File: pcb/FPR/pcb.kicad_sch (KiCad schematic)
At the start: 52 parts, among them J1 Conn_01x03_Male, J12 V Solar, J13 V batt, J2 Conn_01x03_Male, J3 Conn_01x03_Male, J4 Conn_01x03_Male, J5 Conn_01x04_Female, J6 SD Card Reader, J7 cell power headers, J8 cell data headers, U1 ATmega328-P, U2 LM2574HVM-12, U3 LT3650EMSE-8.4-PBF, U4 LM311, Y1 16MHz

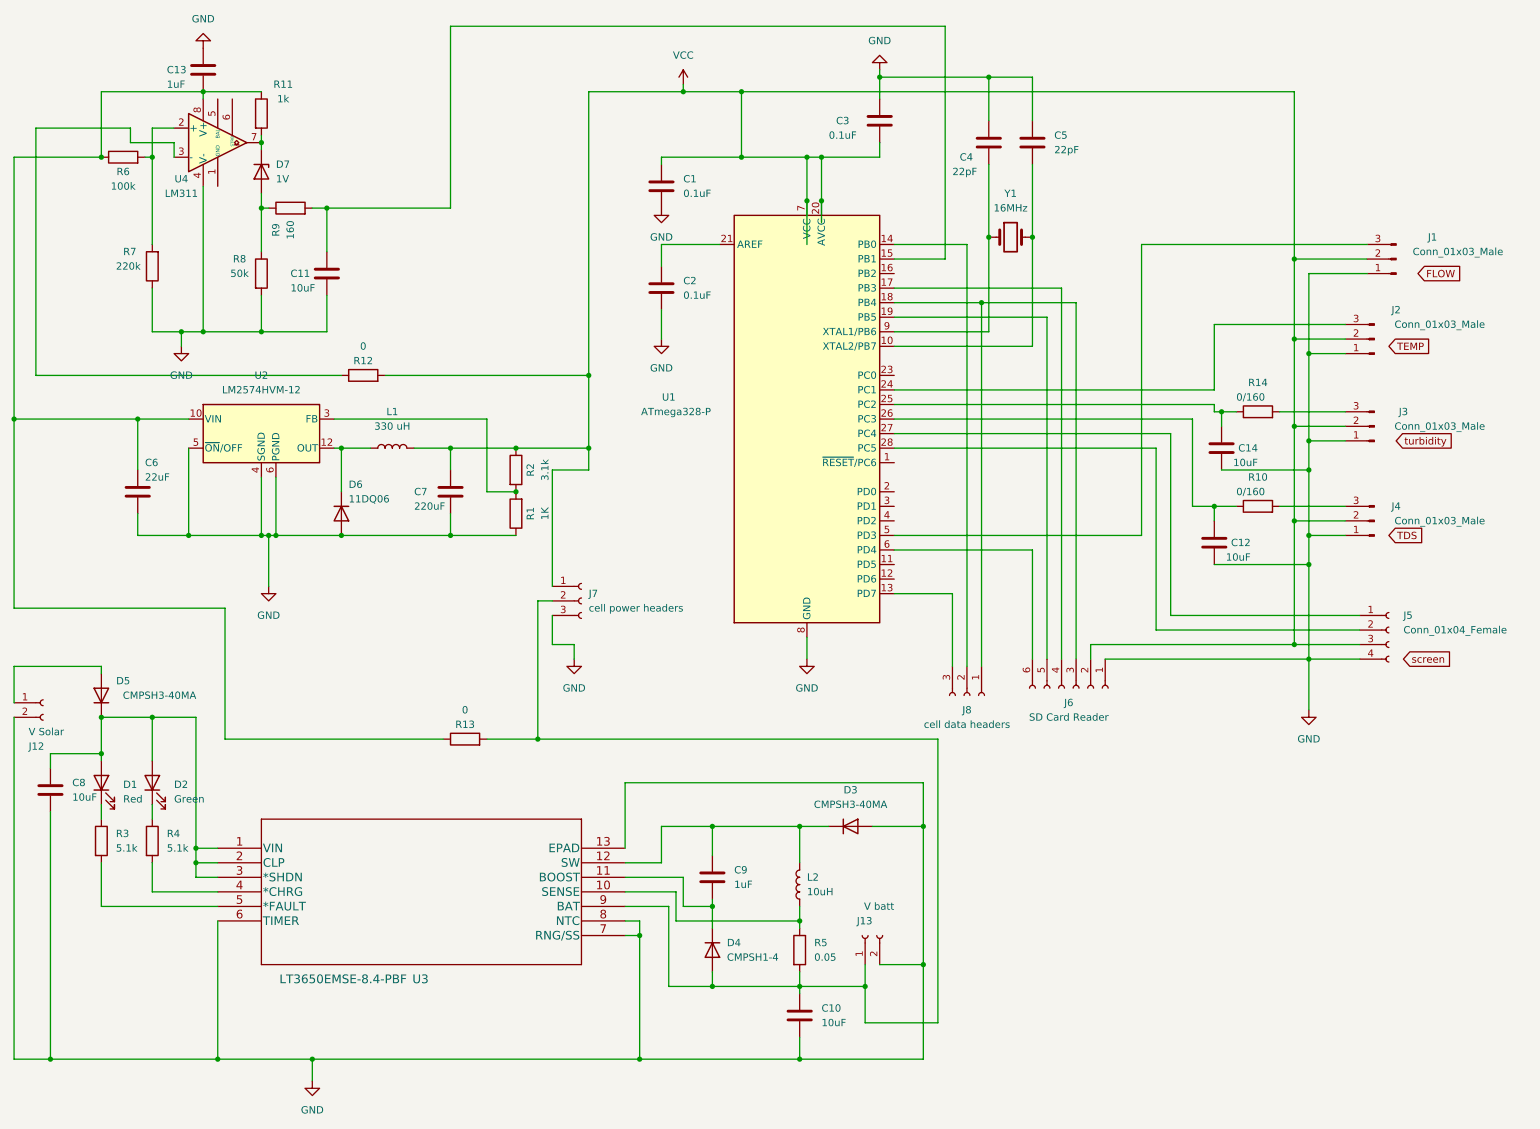
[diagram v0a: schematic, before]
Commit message: recent changes
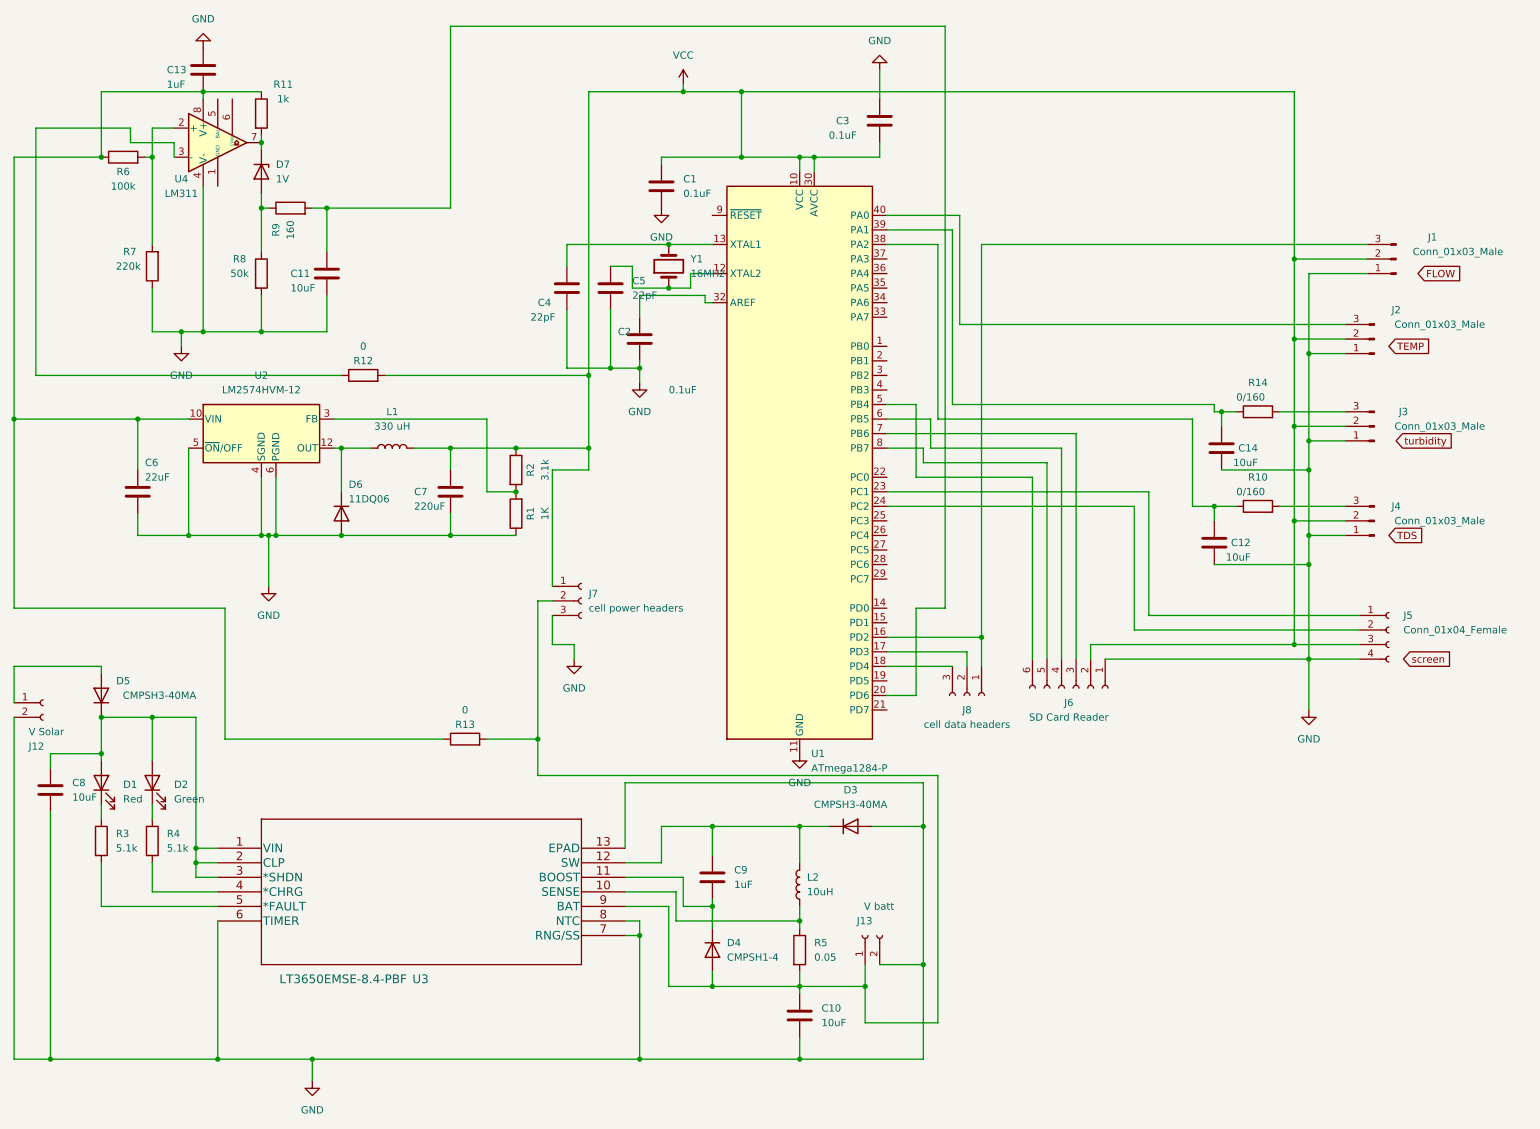
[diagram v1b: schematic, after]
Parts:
- removed U1: ATmega328-P, Package_DIP:DIP-28_W7.62mm_Socket, symbol MCU_Microchip_ATmega:ATmega328-P
- added U1: ATmega1284-P, Package_DIP:DIP-40_W15.24mm, symbol MCU_Microchip_ATmega:ATmega1284-P
- J7: footprint (none) -> Connector_PinHeader_2.54mm:PinHeader_1x03_P2.54mm_Vertical
- J8: footprint Connector_PinSocket_2.54mm:PinSocket_1x03_P2.54mm_Vertical -> Connector_PinHeader_2.54mm:PinHeader_1x03_P2.54mm_Vertical
- L2: footprint Inductor_SMD:L_1206_3216Metric -> Inductor_SMD:L_Bourns-SRN8040_8x8.15mm
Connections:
- net GND: now also C4.2, C5.2, U1.11 (GND), U1.31 (GND); no longer C4.1, C5.1
- net VCC: now also U1.10 (VCC), U1.30 (AVCC)
- net at C2.1: now also U1.32 (AREF)
- net at J6.3 (Pin_3): now also U1.7 (PB6); no longer J8.1 (Pin_1)
- net at J6.4 (Pin_4): now also U1.6 (PB5)
- net at J6.5 (Pin_5): now also U1.8 (PB7)
- net at J6.6 (Pin_6): now also U1.5 (PB4)
- net at J2.3 (Pin_3): now also U1.40 (PA0)
- net at C14.2, R14.1: now also U1.39 (PA1)
- net at Y1.1: now also C5.1, U1.12 (XTAL2); no longer C4.2
- net at Y1.2: now also C4.1, U1.13 (XTAL1); no longer C5.2
- net at C11.1, R9.2: now also U1.20 (PD6)
- net at C12.2, R10.1: now also U1.38 (PA2)
- net at J8.2 (Pin_2): now also U1.17 (PD3)
- net at J8.3 (Pin_3): now also U1.18 (PD4)
- net at J5.1 (Pin_1): now also U1.23 (PC1)
- net at J5.2 (Pin_2): now also U1.24 (PC2)
- net at J1.3 (Pin_3): now also J8.1 (Pin_1), U1.16 (PD2)
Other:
- moved on the sheet: C2
